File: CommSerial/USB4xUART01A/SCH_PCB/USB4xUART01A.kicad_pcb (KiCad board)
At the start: 2 copper layers, 70.6 x 40.1 mm, 94 parts, among them J1 JUMP_2x1, J10 JUMP_2x1, J11 JUMP_2x1, J12 JUMP_2x1, J13 JUMP_2x1, J14 JUMP_2x1, J15 JUMP_2x1, J16 JUMP_2x1, J17 JUMP_2x1, J18 JUMP_2x1, J19 JUMP_2x1, J2 JUMP_2x1, J20 JUMP_2x1, J21 JUMP_2x1, J22 JUMP_2x1, J23 JUMP_2x1, J24 JUMP_2x1, J25 JUMP_2x1, J26 JUMP_2x1, J27 JUMP_2x1, J28 JUMP_2x1, J29 JUMP_2x1, J3 JUMP_2x1, J30 JUMP_2x1, J31 JUMP_2x1, J32 JUMP_2x1, J33 JUMP_2x1, J34 JUMP_2x1, J35 JUMP_3X2, J36 JUMP_3X2, J4 JUMP_2x1, J5 JUMP_2x1, J6 JUMP_2x1, J7 JUMP_2x1, J8 JUMP_2x1, J9 JUMP_2x1, M1 HOLE, M2 HOLE, M3 HOLE, M4 HOLE, P1 USB_B, U1 93LC56BT-I/OT, U2 FT4232HL, U3 LM1117_3V3, U4 SN74HC595D, Y1 12MHz

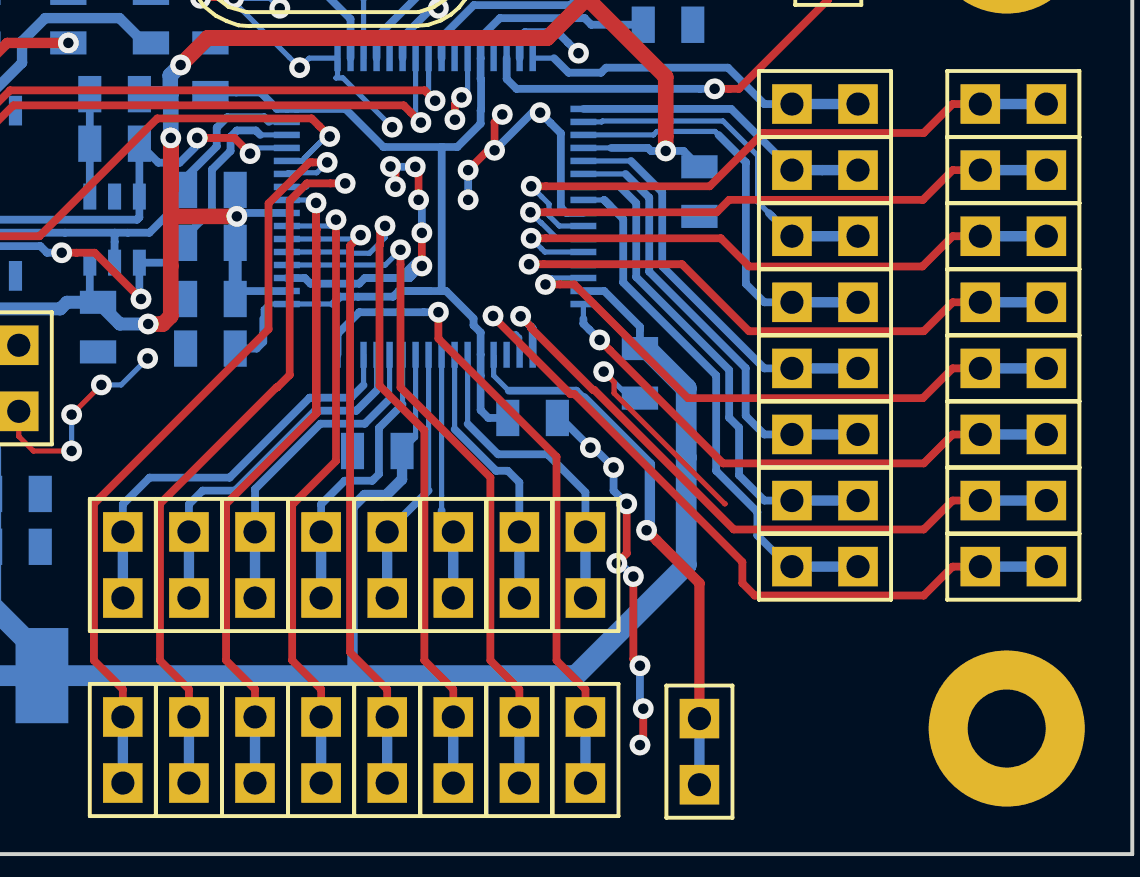
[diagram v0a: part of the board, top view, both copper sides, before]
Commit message: zmena
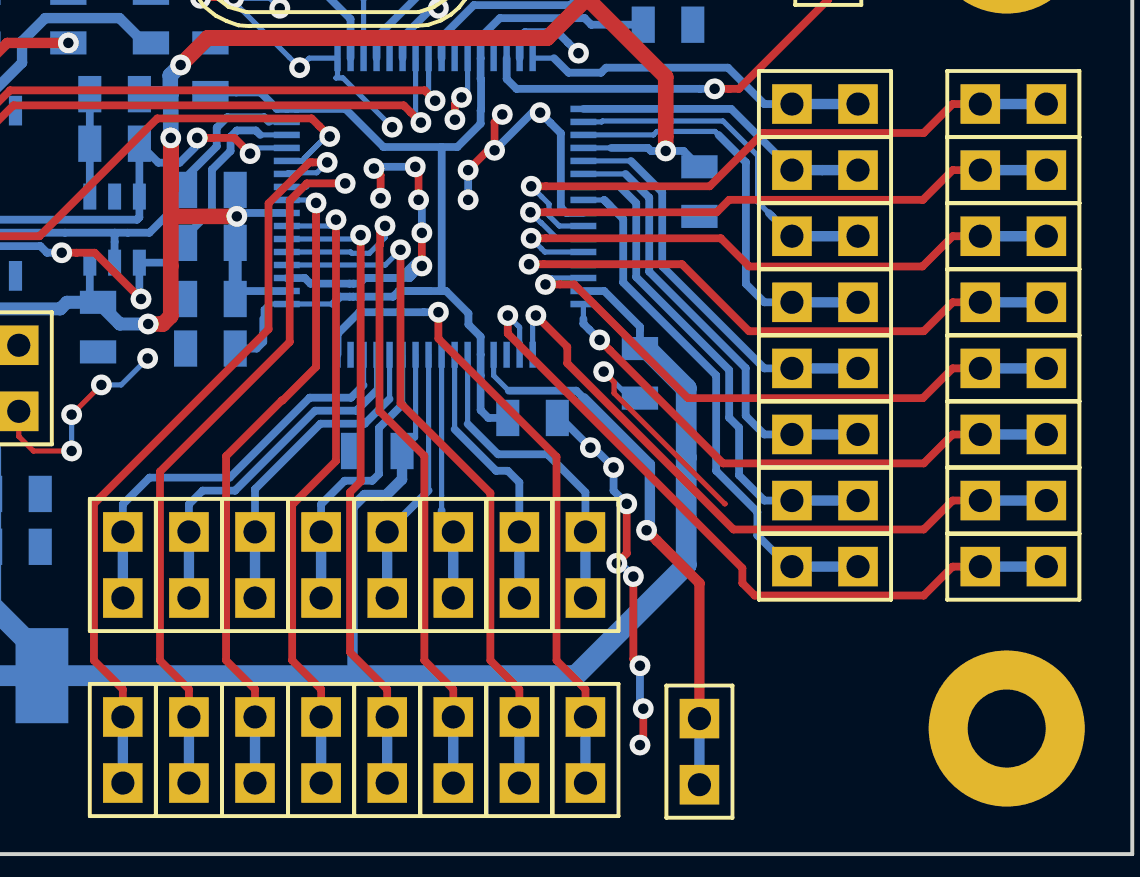
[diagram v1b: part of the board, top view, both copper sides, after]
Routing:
- net /D_DSR: track 33.4 -> 25.4 mm
- net GND: track 101.0 -> 102.0 mm
- net /B_RI: track 28.7 -> 28.1 mm

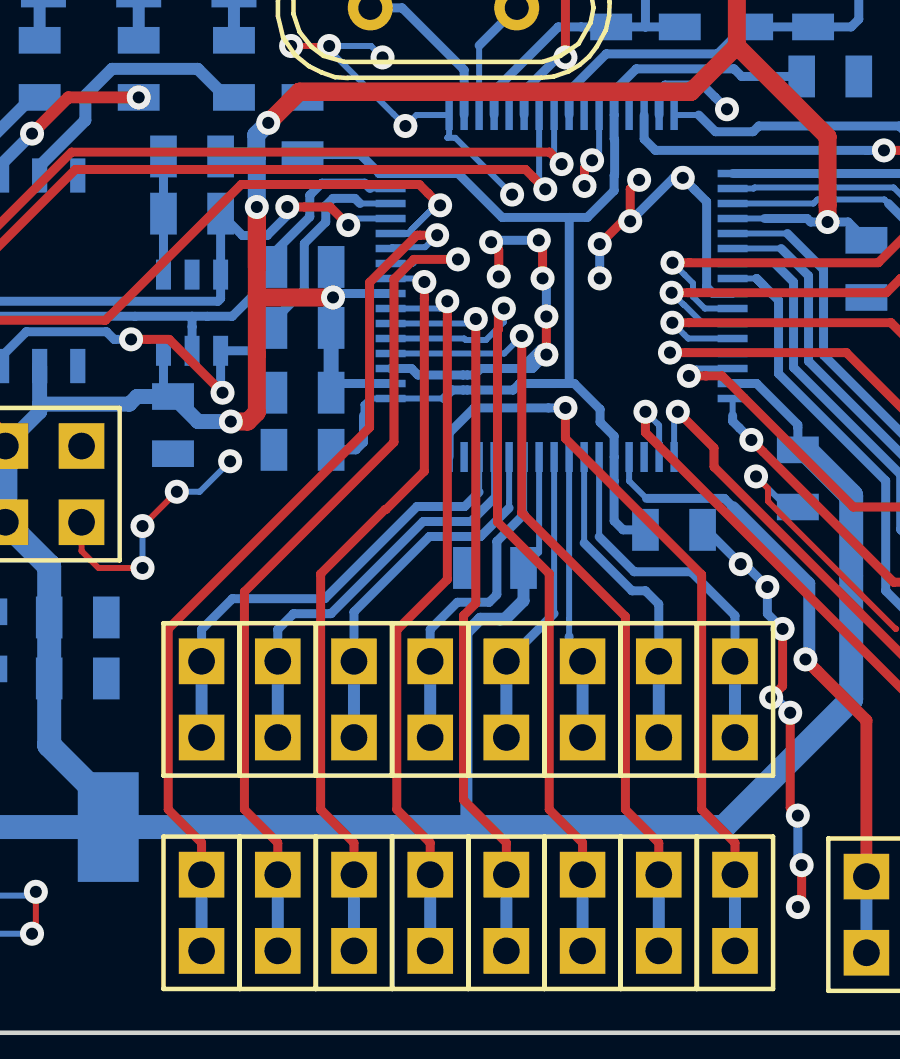
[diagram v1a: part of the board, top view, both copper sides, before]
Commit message: zmena
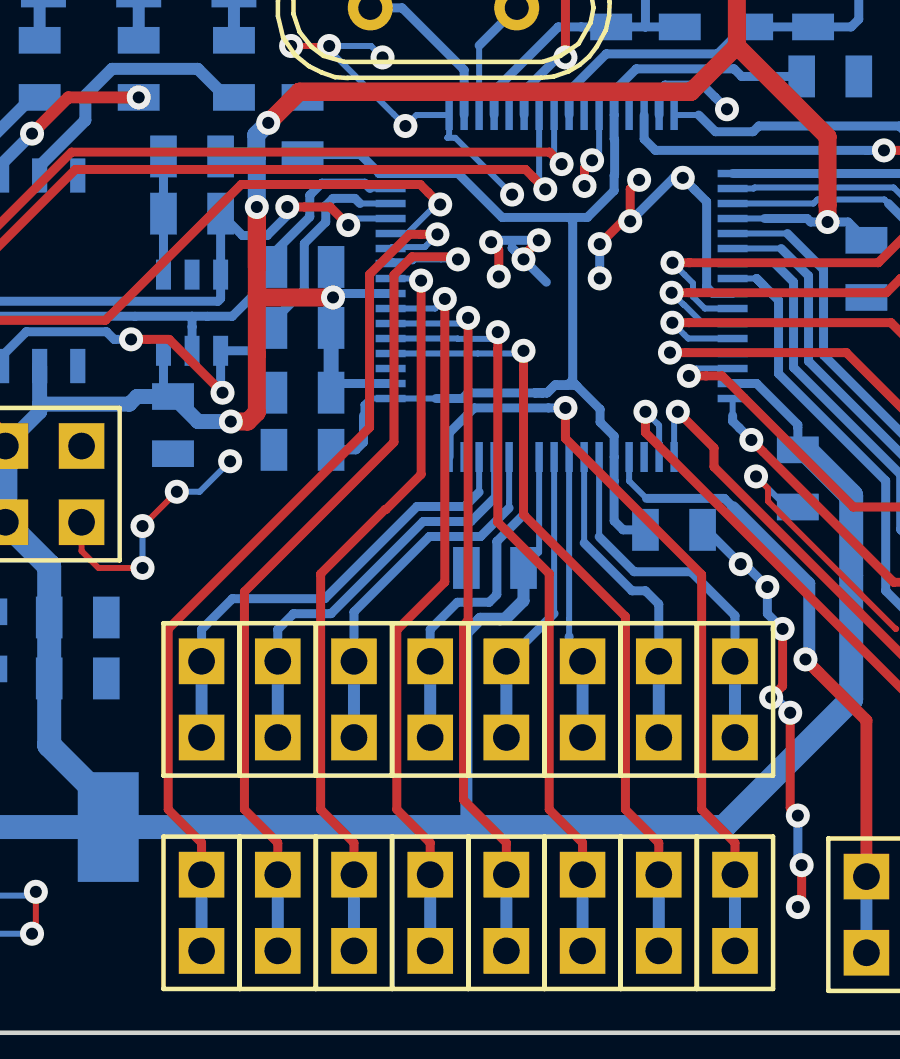
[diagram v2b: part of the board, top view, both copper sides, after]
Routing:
- net GND: track 102.0 -> 87.4 mm, vias 44 -> 38
- net (no net): track 0.00 -> 5.86 mm, vias 0 -> 4
- net /#PWREN: track 28.9 -> 26.1 mm
- net /D_RTS: track 27.2 -> 25.5 mm
- net /D_RXD: track 27.0 -> 26.3 mm
